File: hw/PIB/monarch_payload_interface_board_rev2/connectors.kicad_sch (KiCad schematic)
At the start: 20 parts, among them J1 5037630291, J10 5037630491, J101 Conn_01x03, J102 Conn_01x04, J104 Conn_01x02, J105 Conn_01x02, J106 Conn_01x04, J11 5037630691, J12 5037630691, J13 5037630491, J14 5037630491, J15 5037630691, J2 5037630291, J3 5037630691, J4 5037630691, J5 5037630691, J6 5037630691, J7 5037630691, J8 5037630691, J9 5037630491

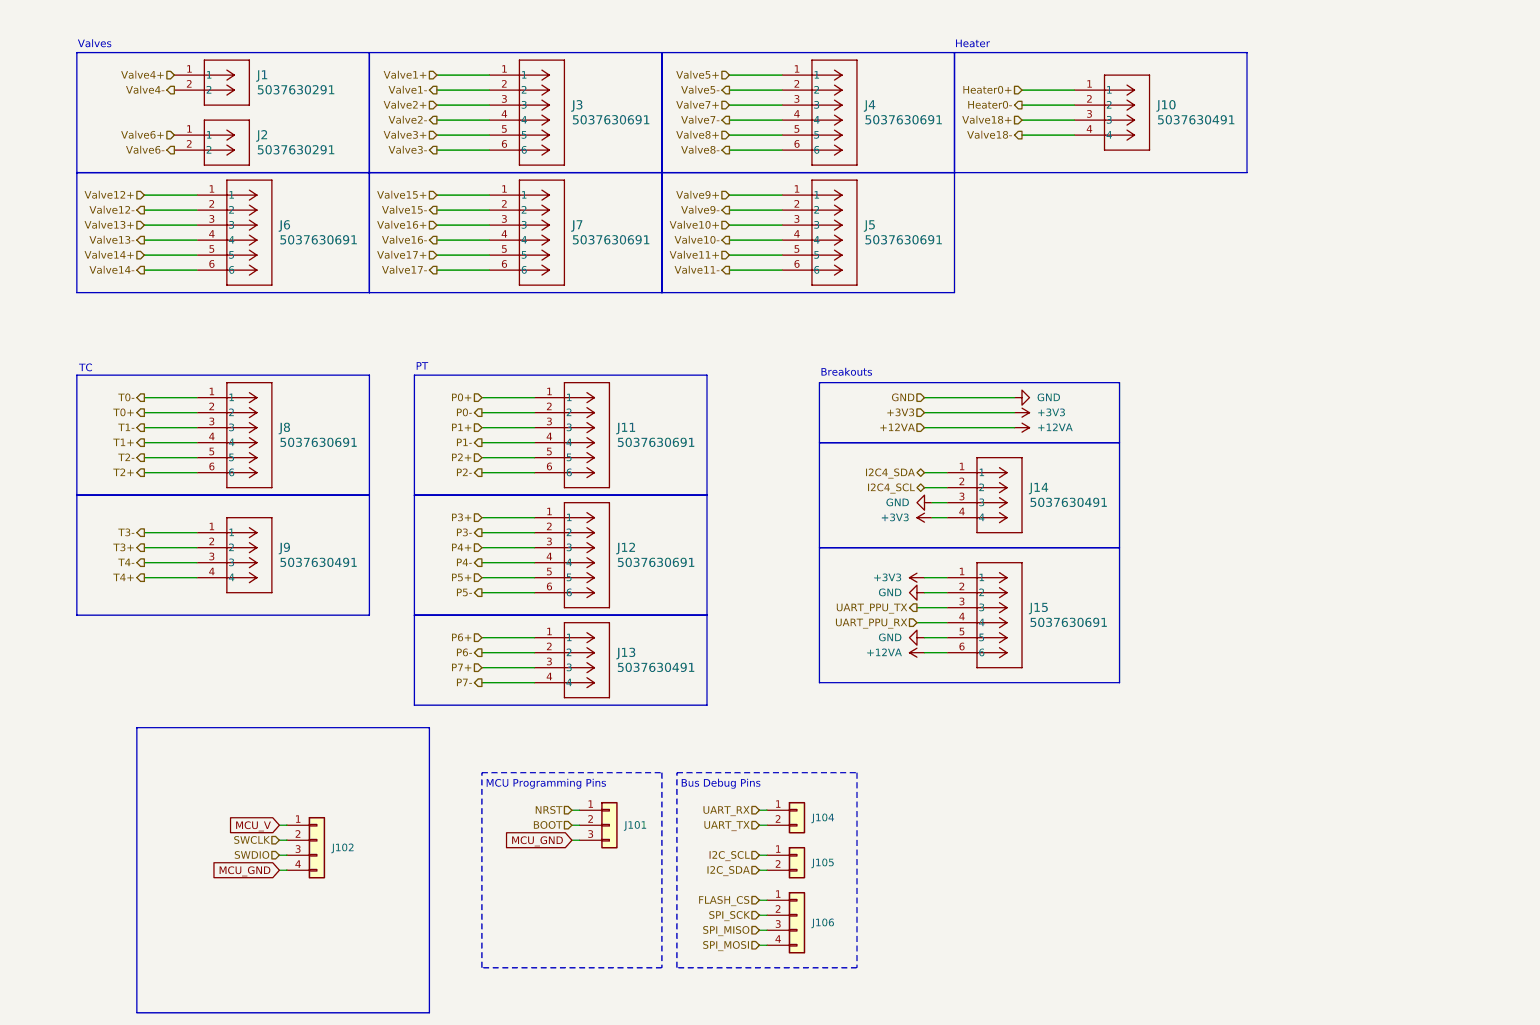
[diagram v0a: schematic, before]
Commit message: Connector Additions
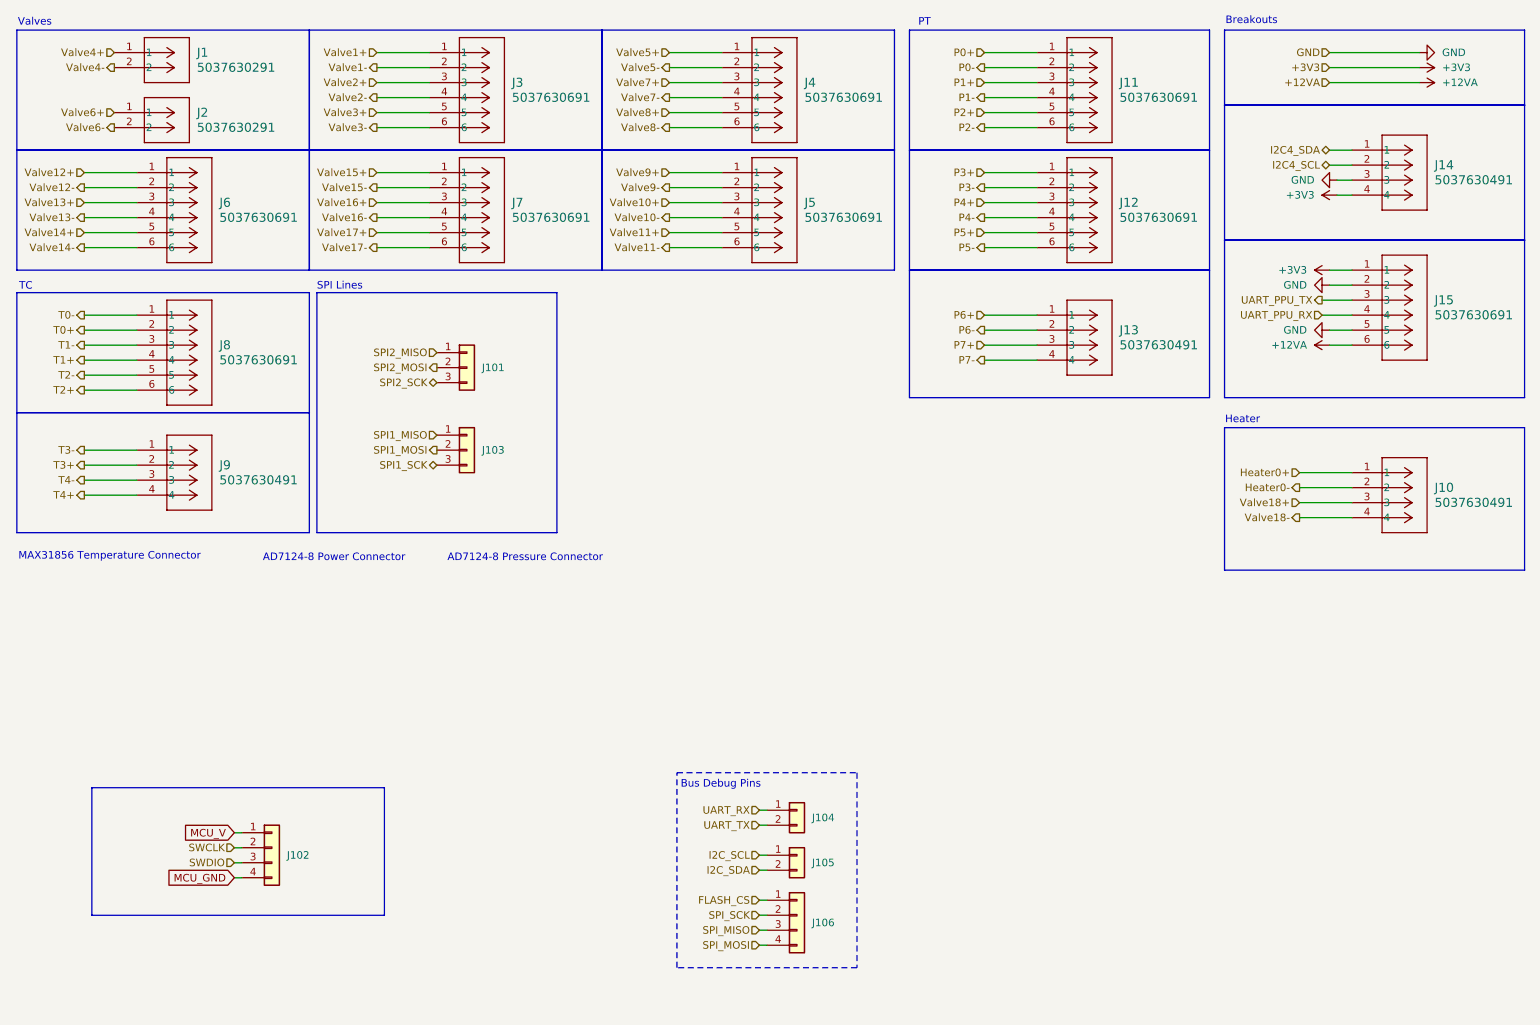
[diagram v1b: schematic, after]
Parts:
- added J103: Conn_01x03, Connector_PinHeader_1.27mm:PinHeader_1x03_P1.27mm_Vertical, symbol Connector_Generic:Conn_01x03
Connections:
- net MCU_GND: no longer J101.3 (Pin_3)
- net BOOT renamed SPI2_MOSI
- net NRST renamed SPI2_MISO
- new net SPI1_MISO: J103.1 (Pin_1)
- new net SPI1_MOSI: J103.2 (Pin_2)
- new net SPI1_SCK: J103.3 (Pin_3)
- new net SPI2_SCK: J101.3 (Pin_3)
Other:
- note added: "AD7124-8 Power Connector"
- note added: "AD7124-8 Pressure Connector"
- note added: "MAX31856 Temperature Connector"
- note added: "SPI Lines"
- note removed: "MCU Programming Pins"
- moved on the sheet: J1, J10, J101, J102, J11, J12, J13, J14, J15, J2, J3, J4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
